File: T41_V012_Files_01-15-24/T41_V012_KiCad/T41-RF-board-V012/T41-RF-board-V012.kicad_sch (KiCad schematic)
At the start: 232 parts, among them J1 IQ_Out, J2 RF_IN, J3 RFControl, J4 12-13.8V, J5 IQ_In, J6 RF_OUT, Q1 BS170, U1 74CBTLV3253DR, U10 SN74LVC1G04DCK, U106 MC33078, U107 MC33078, U11 Si5351A-B-GT, U12 PE4312, U13 MAR-3SM+, U14 LM7805CT, U15 LM1117T-3.3, U16 LM358B, U17 LM317L, U18 SN74LVC1G04DCK, U19 MASWSS0179, U2 PSA-8A+, U20 MASWSS0179, U21 MCP23017_SO, U22 HMC434E, U23 HMC434E, U3 PE4312, U4 74CBTLV3253DR, U5 SN74LVC1G04DCK, U6 MC33078, U7 MASWSS0179, U8 MC33078, U9 MASWSS0179, Y1 ECS-TX053-S3, Y2 25MHz

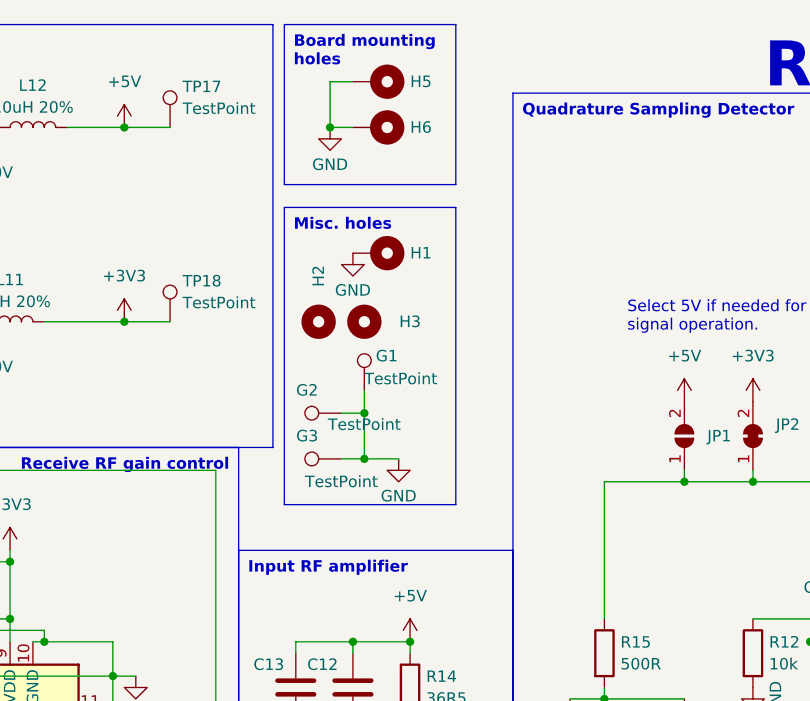
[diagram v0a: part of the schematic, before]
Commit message: Added heatsink model to RF board to confirm component fit. Tweaked locations of a few components.
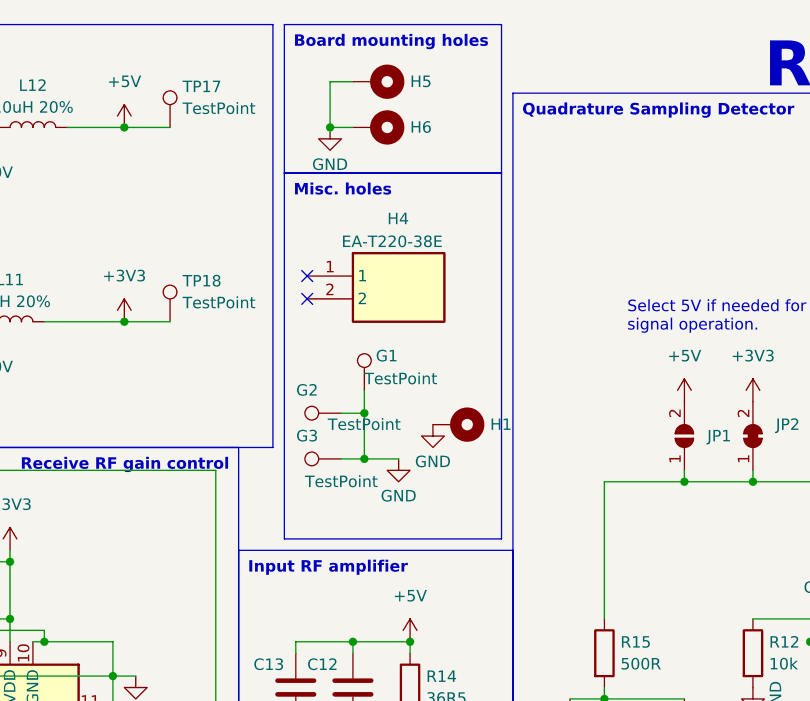
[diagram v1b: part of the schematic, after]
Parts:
- removed H2, H3: ~, MountingHole:MountingHole_3mm_Pad, symbol Mechanical:MountingHole
- added H4: EA-T220-38E, EAT22038E, symbol T41_Library:EA-T220-38E
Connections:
- no-connect marks 12 -> 14
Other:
- moved on the sheet: H1
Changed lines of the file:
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@@
   )
   (no_connect (at 26.67 220.98))
+  (no_connect (at 135.89 43.18))
   (no_connect (at 93.98 144.78))
   (no_connect (at 93.98 167.64))
@@
   (no_connect (at 393.7 66.04))
   (no_connect (at 393.7 71.12))
+  (no_connect (at 135.89 40.64))
   (no_connect (at 156.21 156.21))
   (no_connect (at 93.98 147.32))
@@
   )
   (text_box "Misc. holes"
-    (at 133.35 33.02 0) (size 19.05 33.02)
+    (at 133.35 29.21 0) (size 24.13 40.64)
     (stroke (width 0) (type default))
     (fill (type none))
@@
   )
   (text_box "Board mounting holes"
-    (at 133.35 12.7 0) (size 19.05 17.78)
+    (at 133.35 12.7 0) (size 24.13 16.51)
     (stroke (width 0) (type default))
     (fill (type none))
@@
     )
   )
-  (symbol (lib_id "Mechanical:MountingHole") (at 137.16 45.72 0) (unit 1)
-    (in_bom yes) (on_board yes) (dnp no)
-    (property "Reference" "H2" (at 137.16 40.64 90)
-      (effects (font (size 1.27 1.27)))
-    )
-    (property "Value" "~" (at 139.7 46.9321 0)
-      (effects (font (size 1.27 1.27)) (justify left))
-    )
-    (property "Footprint" "MountingHole:MountingHole_3mm_Pad" (at 137.16 45.72 0)
-      (effects (font (size 1.27 1.27)) hide)
-    )
-    (property "Datasheet" "~" (at 137.16 45.72 0)
-      (effects (font (size 1.27 1.27)) hide)
-    )
-    (property "Mouser" "" (at 137.16 45.72 0)
-      (effects (font (size 1.27 1.27)) hide)
-    )
-    (property "Tayda" "" (at 137.16 45.72 0)
-      (effects (font (size 1.27 1.27)) hide)
-    )
-    (property "PJRC.com" "" (at 137.16 45.72 0)
-      (effects (font (size 1.27 1.27)) hide)
-    )
-    (instances
-      (project "T41-RF-board-V012"
-        (path "/3c4b9d3b-a516-4fd7-b325-b74c836dee65"
-          (reference "H2") (unit 1)
-        )
-      )
-    )
-  )
   (symbol (lib_id "T41_Library:ECS-TX053-S3") (at 368.3 147.32 0) (mirror y) (unit 1)
     (in_bom yes) (on_board yes) (dnp no)
@@
     )
   )
-  (symbol (lib_id "Mechanical:MountingHole") (at 142.24 45.72 270) (unit 1)
-    (in_bom yes) (on_board yes) (dnp no)
-    (property "Reference" "H3" (at 147.32 45.72 90)
-      (effects (font (size 1.27 1.27)))
-    )
-    (property "Value" "~" (at 141.0279 48.26 0)
-      (effects (font (size 1.27 1.27)) (justify left))
-    )
-    (property "Footprint" "MountingHole:MountingHole_3mm_Pad" (at 142.24 45.72 0)
-      (effects (font (size 1.27 1.27)) hide)
-    )
-    (property "Datasheet" "~" (at 142.24 45.72 0)
-      (effects (font (size 1.27 1.27)) hide)
-    )
-    (property "Mouser" "" (at 142.24 45.72 0)
-      (effects (font (size 1.27 1.27)) hide)
-    )
-    (property "Tayda" "" (at 142.24 45.72 0)
-      (effects (font (size 1.27 1.27)) hide)
-    )
-    (property "PJRC.com" "" (at 142.24 45.72 0)
-      (effects (font (size 1.27 1.27)) hide)
-    )
-    (instances
-      (project "T41-RF-board-V012"
-        (path "/3c4b9d3b-a516-4fd7-b325-b74c836dee65"
-          (reference "H3") (unit 1)
-        )
-      )
-    )
-  )
   (symbol (lib_id "Device:L") (at 171.45 191.77 0) (mirror y) (unit 1)
     (in_bom yes) (on_board yes) (dnp no) (fields_autoplaced)
@@
     )
   )
-  (symbol (lib_id "power:GND") (at 140.97 38.1 0) (unit 1)
+  (symbol (lib_id "power:GND") (at 149.86 57.15 0) (unit 1)
     (in_bom yes) (on_board yes) (dnp no) (fields_autoplaced)
-    (property "Reference" "#PWR022" (at 140.97 44.45 0)
+    (property "Reference" "#PWR022" (at 149.86 63.5 0)
       (effects (font (size 1.27 1.27)) hide)
     )
-    (property "Value" "GND" (at 140.97 42.2331 0)
+    (property "Value" "GND" (at 149.86 61.2831 0)
       (effects (font (size 1.27 1.27)))
     )
-    (property "Footprint" "" (at 140.97 38.1 0)
+    (property "Footprint" "" (at 149.86 57.15 0)
       (effects (font (size 1.27 1.27)) hide)
     )
-    (property "Datasheet" "" (at 140.97 38.1 0)
+    (property "Datasheet" "" (at 149.86 57.15 0)
       (effects (font (size 1.27 1.27)) hide)
     )
@@
     )
   )
+  (symbol (lib_id "T41_Library:EA-T220-38E") (at 135.89 40.64 0) (unit 1)
+    (in_bom yes) (on_board yes) (dnp no)
+    (property "Reference" "H4" (at 144.78 34.29 0)
+      (effects (font (size 1.27 1.27)) (justify left))
+    )
+    (property "Value" "EA-T220-38E" (at 139.7 36.83 0)
+      (effects (font (size 1.27 1.27)) (justify left))
+    )
+    (property "Footprint" "EAT22038E" (at 152.4 135.56 0)
+      (effects (font (size 1.27 1.27)) (justify left top) hide)
+    )
+    (property "Datasheet" "https://www.ohmite.com/assets/docs/sink_e.pdf?r=false" (at 152.4 235.56 0)
+      (effects (font (size 1.27 1.27)) (justify left top) hide)
+    )
+    (property "Height" "38.35" (at 152.4 435.56 0)
+      (effects (font (size 1.27 1.27)) (justify left top) hide)
+    )
+    (property "Mouser Part Number" "588-EA-T220-38E" (at 152.4 535.56 0)
+      (effects (font (size 1.27 1.27)) (justify left top) hide)
+    )
+    (property "Mouser Price/Stock" "https://www.mouser.co.uk/ProductDetail/Ohmite/EA-T220-38E?qs=6weo7U0lPxCX9kcQhGcuZQ%3D%3D" (at 152.4 635.56 0)
+      (effects (font (size 1.27 1.27)) (justify left top) hide)
+    )
+    (property "Manufacturer_Name" "Ohmite" (at 152.4 735.56 0)
+      (effects (font (size 1.27 1.27)) (justify left top) hide)
+    )
+    (property "Manufacturer_Part_Number" "EA-T220-38E" (at 152.4 835.56 0)
+      (effects (font (size 1.27 1.27)) (justify left top) hide)
+    )
+    (pin "1")
+    (pin "2")
+    (instances
+      (project "T41-RF-board-V012"
+        (path "/3c4b9d3b-a516-4fd7-b325-b74c836dee65"
+          (reference "H4") (unit 1)
+        )
+      )
+    )
+  )
   (symbol (lib_id "Amplifier_Operational:MC33078") (at 99.06 205.74 0) (mirror x) (unit 2)
     (in_bom yes) (on_board yes) (dnp no)
@@
     )
   )
-  (symbol (lib_id "Mechanical:MountingHole_Pad") (at 143.51 38.1 270) (unit 1)
+  (symbol (lib_id "Mechanical:MountingHole_Pad") (at 152.4 57.15 270) (unit 1)
     (in_bom no) (on_board yes) (dnp no) (fields_autoplaced)
-    (property "Reference" "H1" (at 147.32 38.1 90)
+    (property "Reference" "H1" (at 156.21 57.15 90)
       (effects (font (size 1.27 1.27)) (justify left))
     )
-    (property "Value" "~" (at 147.32 39.3121 90)
+    (property "Value" "~" (at 156.21 58.3621 90)
       (effects (font (size 1.27 1.27)) (justify left))
     )
-    (property "Footprint" "MountingHole:MountingHole_3.2mm_M3_Pad" (at 143.51 38.1 0)
+    (property "Footprint" "MountingHole:MountingHole_3.2mm_M3_Pad" (at 152.4 57.15 0)
       (effects (font (size 1.27 1.27)) hide)
     )
-    (property "Datasheet" "~" (at 143.51 38.1 0)
+    (property "Datasheet" "~" (at 152.4 57.15 0)
       (effects (font (size 1.27 1.27)) hide)
     )
-    (property "Mouser Part Number" "" (at 143.51 38.1 0)
+    (property "Mouser Part Number" "" (at 152.4 57.15 0)
       (effects (font (size 1.27 1.27)) hide)
     )
